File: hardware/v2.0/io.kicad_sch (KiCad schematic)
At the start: 1 part, among them U1 ECP5U-25F-CABGA256

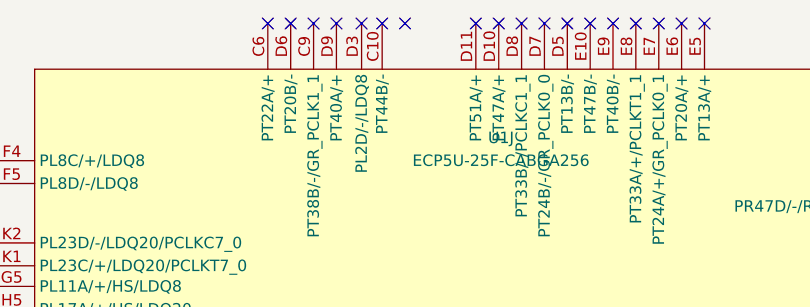
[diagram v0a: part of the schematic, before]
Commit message: DAC Vout
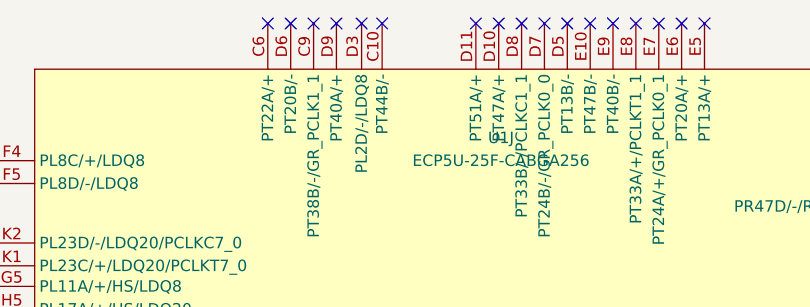
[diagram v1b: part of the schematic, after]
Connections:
- no-connect marks 70 -> 69
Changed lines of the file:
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@@
-	)
-	(no_connect
-		(at 144.526 50.8)
 	)
 	(no_connect
@@
 		(pin "C11"
 		)
+		(pin "E13"
+		)
+		(pin "E12"
+		)
+		(pin "D13"
+		)
 		(instances

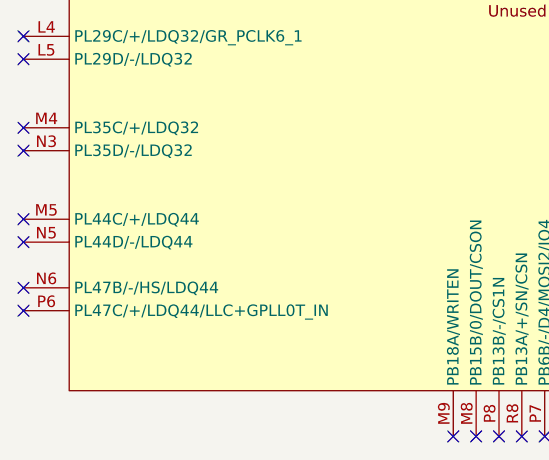
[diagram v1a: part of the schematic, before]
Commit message: ERC pass
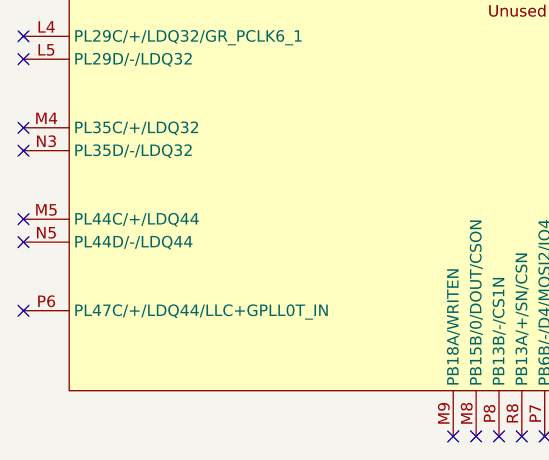
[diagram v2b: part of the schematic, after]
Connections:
- no-connect marks 69 -> 68
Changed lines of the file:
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@@
-	)
-	(no_connect
-		(at 98.298 124.46)
 	)
 	(no_connect
@@
 		(pin "R8"
 		)
-		(pin "E12"
-		)
 		(pin "L2"
 		)
 		(pin "R7"
 		)
-		(pin "E13"
-		)
 		(pin "F13"
 		)
@@
 		(pin "H6"
 		)
-		(pin "N6"
-		)
 		(pin "M5"
 		)
@@
 		(pin "C8"
 		)
-		(pin "D13"
-		)
 		(pin "G2"
